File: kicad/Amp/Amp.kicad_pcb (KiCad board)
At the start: 2 copper layers, 30 x 25.6 mm, 31 parts, among them J1 Conn, J2 Conn, J3 Conn, J4 Conn, J5 Conn, U1 TS5A3166DBVR, U2 MCP1700

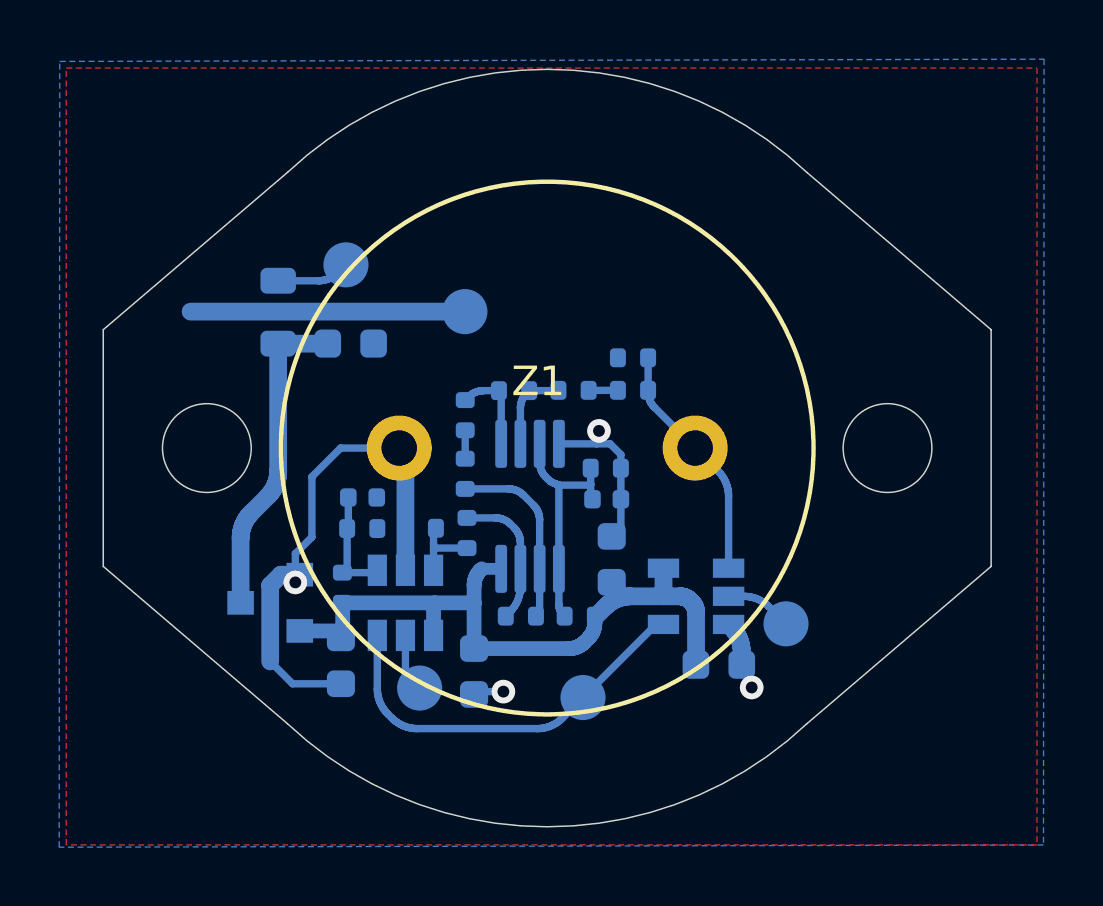
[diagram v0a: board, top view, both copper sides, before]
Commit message: изменено:      kicad/Amp/Amp-cache.lib 	изменено:      kicad/Amp/Amp.kicad_pcb 	изменено:      kicad/Amp/Amp.kicad_pcb-bak 	изменено:      kicad/Amp/Amp.sch 	изменено:      kicad/Amp/Amp.sch-bak
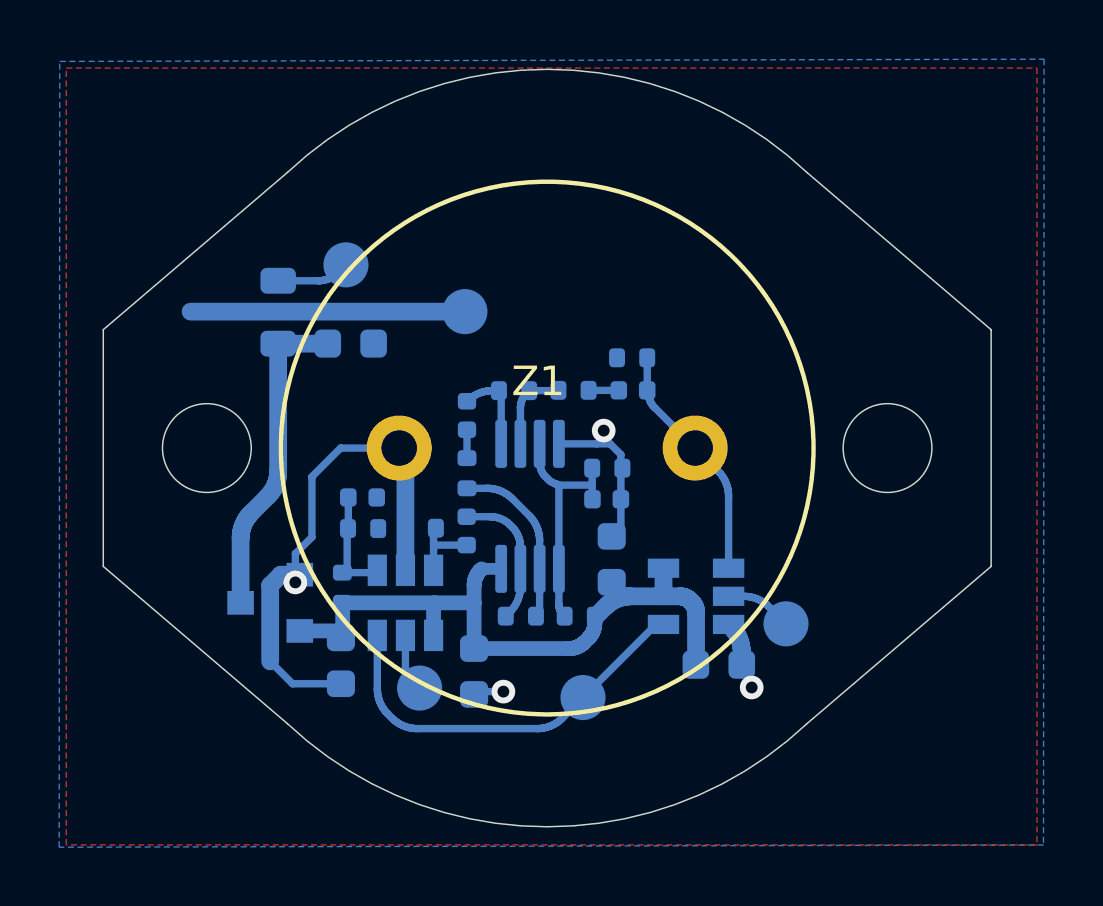
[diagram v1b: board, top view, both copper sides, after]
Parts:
- C2, C4, C6: footprint Resistor_SMD:R_0402_1005Metric -> Capacitor_SMD:C_0402_1005Metric
- moved C6 0.07 mm to (40.3, 80.5)
- moved R6 0.06 mm to (40.3, 78.5)
- moved C4 0.06 mm to (40.3, 76.6)
- moved R4 0.05 mm to (45.0, 78.4)
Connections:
- net Net-(C2-Pad2) renamed /In
